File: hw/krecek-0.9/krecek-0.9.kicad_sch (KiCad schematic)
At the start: 1 part, among them U13 Display

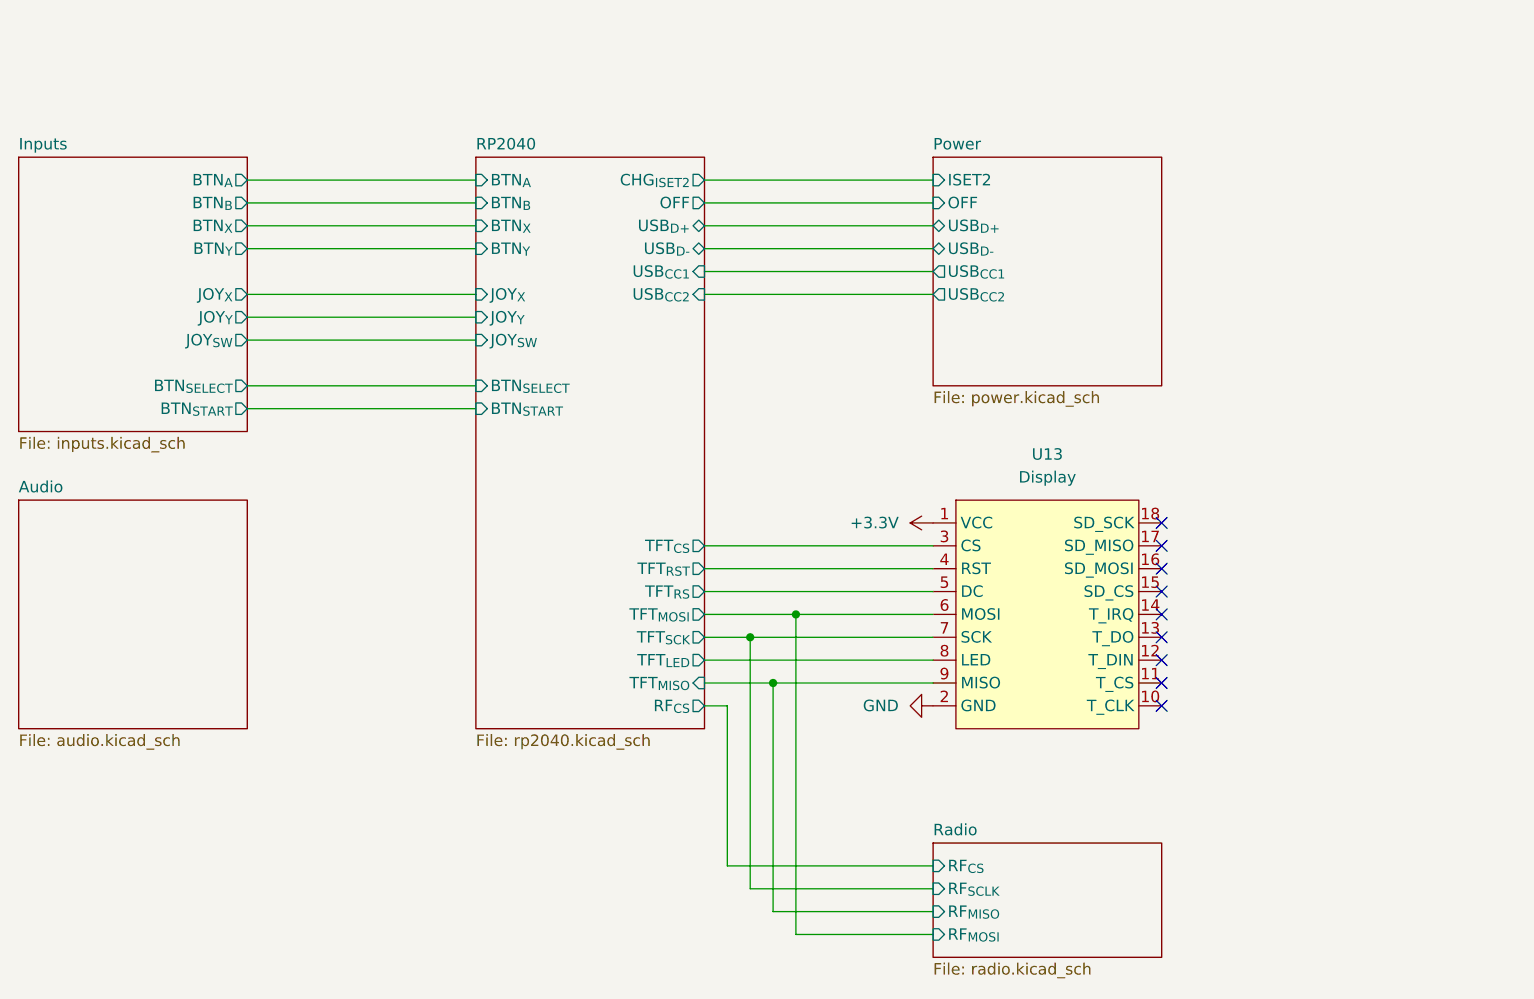
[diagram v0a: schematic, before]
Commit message: Complete most of the design, except for RF
Signed-off-by: Jan Hamal Dvořák <mordae@anilinux.org>
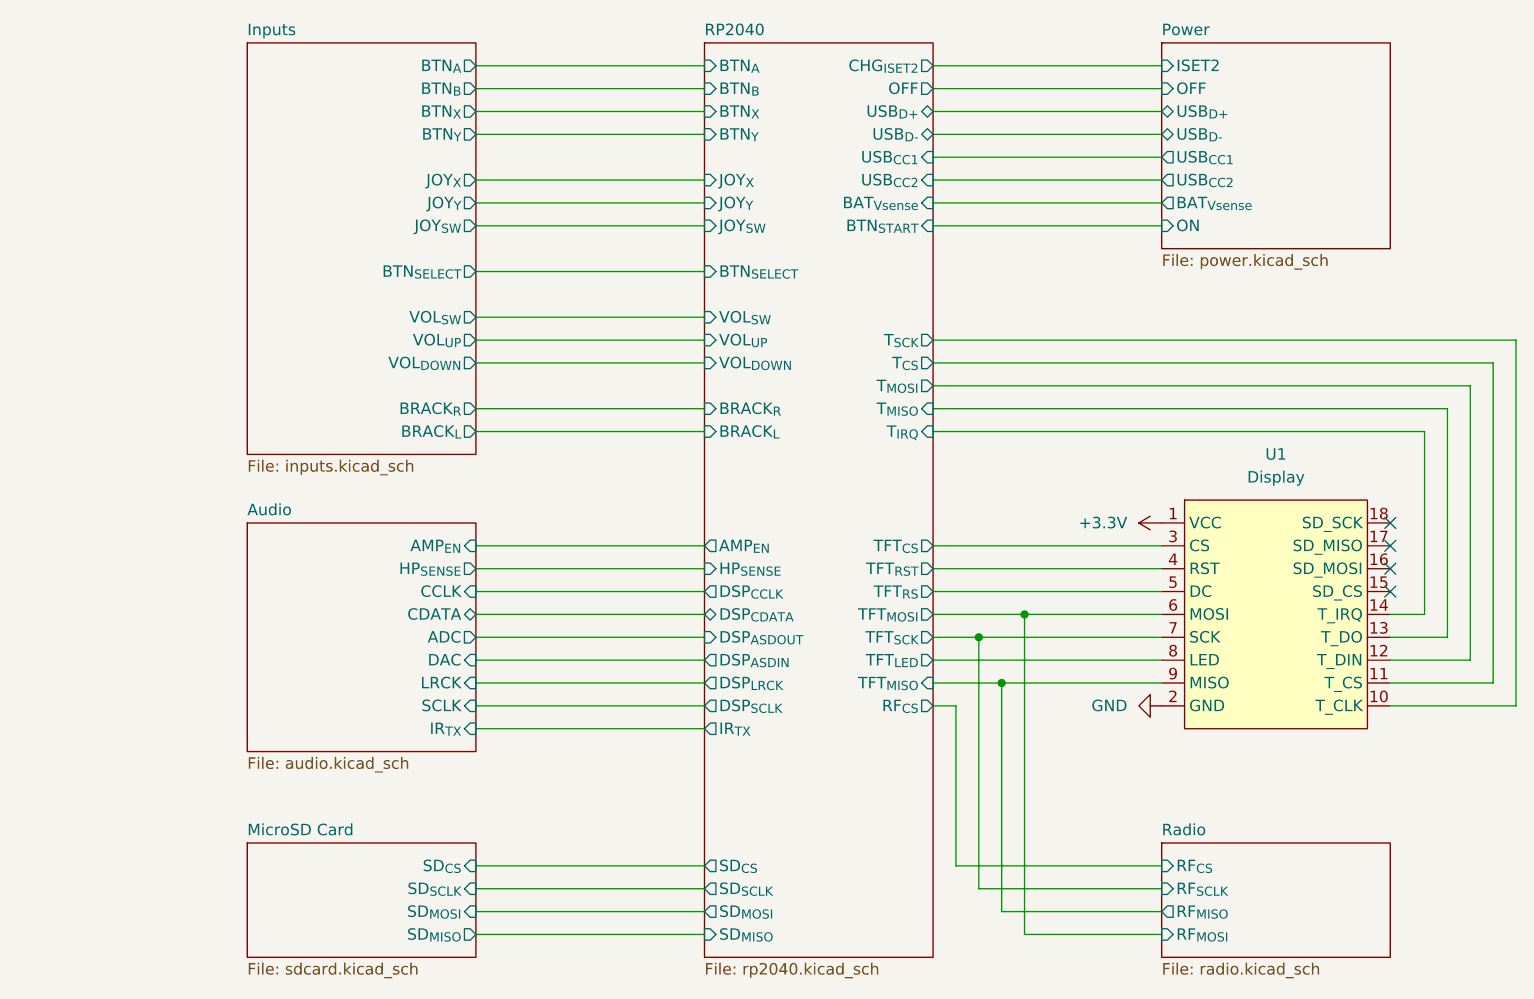
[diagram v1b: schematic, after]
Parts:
- renumbered U13 to U1
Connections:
- net RP2040/T_{SCK}: now reaches U1.10 (T_CLK)
- net RP2040/T_{CS}: now reaches U1.11 (T_CS)
- net RP2040/T_{MOSI}: now reaches U1.12 (T_DIN)
- net RP2040/T_{MISO}: now reaches U1.13 (T_DO)
- net RP2040/T_{IRQ}: now reaches U1.14 (T_IRQ)
- no-connect marks 9 -> 4
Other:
- added sheet MicroSD Card (sdcard.kicad_sch)
- sheet Audio ports: added ADC, AMP_{EN}, CCLK, CDATA, DAC, HP_{SENSE}, IR_{TX}, LRCK, SCLK; removed none
- sheet Inputs ports: added BRACK_{L}, BRACK_{R}, VOL_{DOWN}, VOL_{SW}, VOL_{UP}; removed BTN_{START}
- sheet Power ports: added BAT_{Vsense}, ON; removed none
- sheet RP2040 ports: added AMP_{EN}, BAT_{Vsense}, BRACK_{L}, BRACK_{R}, DSP_{ASDIN}, DSP_{ASDOUT}, DSP_{CCLK}, DSP_{CDATA}, DSP_{LRCK}, DSP_{SCLK}, HP_{SENSE}, IR_{TX}, SD_{CS}, SD_{MISO}, SD_{MOSI}, SD_{SCLK}, T_{CS}, T_{IRQ}, T_{MISO}, T_{MOSI}, T_{SCK}, VOL_{DOWN}, VOL_{SW}, VOL_{UP}; removed none
- moved on the sheet: U1
